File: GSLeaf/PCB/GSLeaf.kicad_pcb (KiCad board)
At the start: 2 copper layers, 30 x 103 mm, 119 parts, among them Q1 LED_5050, Q2 IRLML6401, Q3 IRLML6401, Q4 IRLML9303, Q5 2N7002, SW1 SWITCH, SW2 BTN, SW3 BTN, SW4 DIPx6

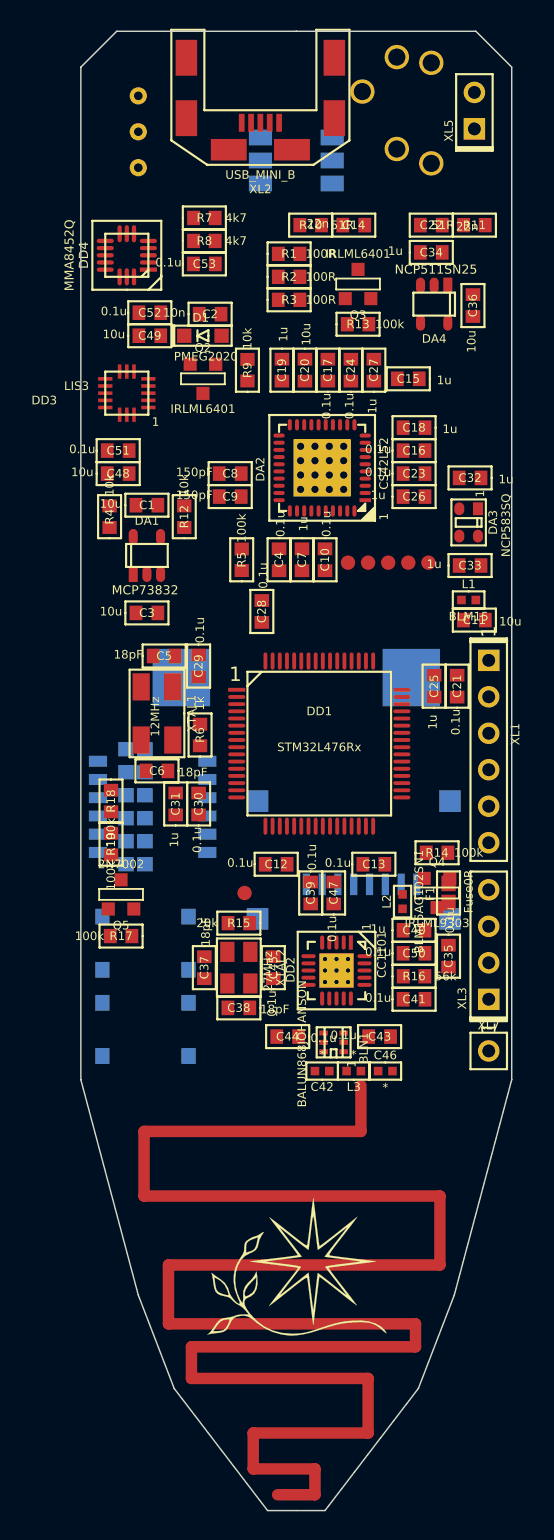
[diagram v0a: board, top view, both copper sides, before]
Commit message: Leaf sent to factory
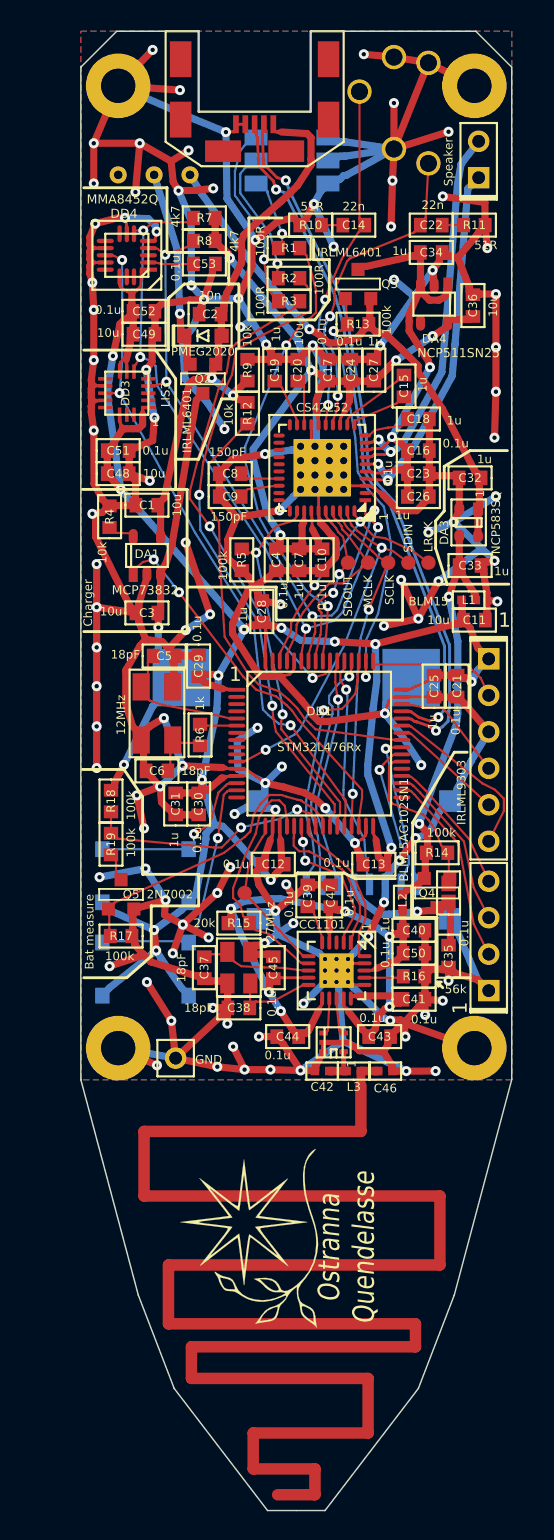
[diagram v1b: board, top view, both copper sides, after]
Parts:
- removed F2, F3, F4, F5, F6, F7: Fuse0R, Resistors:RES_0603_FUSE
- removed SW4: DIPx6, BtnsSwitches:DIP_SMD_1D27X6
- added HOLE1: HOLE_METALLED, PCB:Hole2d4_out4d5mm, F.Cu at (130.6, 61.8)
- added HOLE2: HOLE_METALLED, PCB:Hole2d4_out4d5mm, F.Cu at (130.6, 128.8)
- added HOLE3: HOLE_METALLED, PCB:Hole2d4_out4d5mm, F.Cu at (155.4, 61.8)
- added HOLE4: HOLE_METALLED, PCB:Hole2d4_out4d5mm, F.Cu at (155.4, 128.8)
- moved XL7 21.8 mm to (134.6, 129.5)
- moved R12 8.44 mm to (139.6, 84.6)
- moved SW2 4.70 mm to (132.5, 116.8), turned to 180 degrees
- moved SW3 4.20 mm to (132.5, 123.3)
- moved Logo1 3.81 mm to (139.7, 142.1), turned to 90 degrees
- moved XL5 3.41 mm to (155.7, 68.2)
- moved SW1 3.20 mm to (133.1, 68.0), turned to 180 degrees
- moved C18 0.67 mm to (151.5, 85.0)
- moved XL3 0.60 mm to (156.4, 124.8)
- moved C15 0.58 mm to (150.5, 82.7), turned to 90 degrees
- moved C19 0.50 mm to (141.5, 81.6)
- moved C20 0.50 mm to (143.1, 81.6)
- moved C49 0.41 mm to (132.4, 79.1)
- moved XL2 0.41 mm to (140.1, 63.6)
- moved C52 0.41 mm to (132.4, 77.5)
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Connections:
- DD1 pad 10: /DS1 -> (no net)
- DD1 pad 2: /DS6 -> (no net)
- DD1 pad 3: /DS5 -> (no net)
- DD1 pad 4: /DS4 -> (no net)
- DD1 pad 8: /DS3 -> (no net)
- DD1 pad 9: /DS2 -> (no net)
- Q1 pad 1: GND -> Net-(Q1-Pad1)
- Q1 pad 2: GND -> Net-(Q1-Pad2)
- Q1 pad 3: GND -> Net-(Q1-Pad3)
- Q1 pad 4: Net-(Q1-Pad4) -> GND
- Q1 pad 5: Net-(Q1-Pad5) -> GND
- Q1 pad 6: Net-(Q1-Pad6) -> GND
- R1 pad 1: Net-(Q1-Pad6) -> Net-(Q1-Pad1)
- R2 pad 1: Net-(Q1-Pad5) -> Net-(Q1-Pad2)
- R3 pad 1: Net-(Q1-Pad4) -> Net-(Q1-Pad3)
- XL2 pad H2: Net-(XL2-PadH1) -> (no net)
- XL2 pad H3: Net-(XL2-PadH3) -> (no net)
- XL2 pad H4: Net-(XL2-PadH3) -> Net-(XL2-PadH4)
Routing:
- net GND: track 0.00 -> 648.1 mm, vias 0 -> 116
- net PwrMCU: track 0.00 -> 158.5 mm, vias 0 -> 13
- net /ANT2: track 0.00 -> 142.0 mm
- net VCC: track 0.00 -> 59.9 mm, vias 0 -> 6
- net VAA: track 0.00 -> 58.3 mm, vias 0 -> 5
- net /SDA: track 0.00 -> 51.0 mm, vias 0 -> 4
- net /D-: track 0.00 -> 48.4 mm, vias 0 -> 2
- net /D+: track 0.00 -> 47.4 mm, vias 0 -> 2
- net /SCL: track 0.00 -> 47.2 mm, vias 0 -> 4
- net /ACC_INT1: track 0.00 -> 46.7 mm, vias 0 -> 3
- net /RED_LED: track 0.00 -> 44.7 mm, vias 0 -> 2
- net /GREEN_LED: track 0.00 -> 42.7 mm, vias 0 -> 2
- net +5V: track 0.00 -> 40.4 mm, vias 0 -> 2
- net PwrUnst: track 0.00 -> 38.1 mm, vias 0 -> 1
- net /PWR_CTRLED: track 0.00 -> 32.7 mm, vias 0 -> 2
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- added copper zone on B.Cu, net GND
- added copper zone on F.Cu, net GND
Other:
- outline, holes or cut-outs redrawn
- net class Default: clearance 0.2 -> 0.15; trace_width 0.25 -> 0.15; via_dia 0.8 -> 0.7; via_drill 0.4 -> 0.3
- net class Wide added: clearance 0.15, trace_width 0.5, via_dia 0.7, via_drill 0.3
- rule pad_to_mask_clearance: 0 -> 0.1
- rule trace_clearance: 0.2 -> 0.15
- rule trace_min: 0.2 -> 0.1
- board text added: "+"
- board text added: "-"
- board text added: "Bat measure"
- board text added: "Charger"
- board text added: "GND"
- board text added: "LRCK"
- board text added: "MCLK"
- board text added: "Off On"
- board text added: "Ostranna Quendelasse"
- board text added: "PB13"
- board text added: "PB14"
- board text added: "PB15"
- board text added: "SCLK"
- board text added: "SDIN"
- board text added: "SDOUT"
- board text added: "Speaker"

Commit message: New leaf sch nearly ready
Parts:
- removed ANT1: ANT_PCB_MONO, Radio:ANT_868_SEIDHE
- removed B1: BAT, Installation:EEMB603030
- removed BLN1: BALUN868JOHANSON, Radio:BALUN_JOHANSON868
- removed C1, C11, C20, C3, C36, C48, C49: 10u, Capacitors:CAP_0603
- removed C10, C12, C13, C16, C17, C21, C23, C24, C28, C29, C30, C35, C39, C4, C41, C43, C44, C45, C47, C50, C51, C52, C53: 0.1u, Capacitors:CAP_0603
- removed C14, C22: 22n, Capacitors:CAP_0603
- removed C15, C18, C19, C25, C26, C27, C31, C32, C33, C34, C40, C7: 1u, Capacitors:CAP_0603
- removed C2: 10n, Capacitors:CAP_0603
- removed C37, C38, C5, C6: 18pF, Capacitors:CAP_0603
- removed C42, C46: *, Capacitors:CAP_0402
- removed C8, C9: 150pF, Capacitors:CAP_0603
- removed D1: PMEG2020, Diodes:SOD323
- removed DA1: MCP73832, SOT:SOT23-5
- removed DA2: CS42L52, QFN_DFN:QFN40
- removed DA3: NCP583SQ, SOT:SC82AB
- removed DA4: NCP511SN25, SOT:SOT23-5
- removed DD1: STM32L476Rx, LQFP_TQFP:LQFP64
- removed DD2: CC1101, QFN_DFN:QFN20
- removed DD3: LIS3, LGA:LGA16_3X3_5_3
- removed DD4: MMA8452Q, QFN_DFN:QFN16_5x3
- removed F1: Fuse0R, Resistors:RES_0603_FUSE
- removed HOLE1, HOLE2, HOLE3, HOLE4: HOLE_METALLED, PCB:Hole2d4_out4d5mm
- removed L1: BLM15, Inductors:IND_0402
- removed L2: BLM15AG102SN1, Inductors:IND_0402
- removed L3: *, Inductors:IND_0402
- removed Logo1: Logo, Pictures:Ostranna_12d7_10d1
- removed Q1: LED_5050, LEDs:LED_5050
- removed Q2, Q3: IRLML6401, SOT:SOT23-3
- removed Q4: IRLML9303, SOT:SOT23-3
- removed Q5: 2N7002, SOT:SOT23-3
- removed R1, R2, R3: 100R, Resistors:RES_0603
- removed R10, R11: 51R, Resistors:RES_0603
- removed R12, R4, R9: 10k, Resistors:RES_0603
- removed R13, R14, R17, R18, R19, R5: 100k, Resistors:RES_0603
- removed R15: 20k, Resistors:RES_0603
- removed R16: 56k, Resistors:RES_0603
- removed R6: 1k, Resistors:RES_0603
- removed R7, R8: 4k7, Resistors:RES_0603
- removed SW1: SWITCH, BtnsSwitches:SW_SS-1P2T
- removed SW2, SW3: BTN, BtnsSwitches:BTN_4x4_SMD
- removed TP2, TP3, TP4, TP5, TP6, TP7: TESTPOINT, PCB:TESTPOINT_1MM
- removed XL1: CONN_6, Connectors:PLS-6
- removed XL2: USB_MINI_B, Connectors:USBmicro_MOLEX_WM17142
- removed XL3: CONN_4, Connectors:PLS-4
- removed XL4: AudioJackSimple, Connectors:AUDIO_CKX3_5_30
- removed XL5: CONN_2, Connectors:PLS-2
- removed XL6: CONN_MICROSD, Connectors:MICROSD_CAP_FIX05A
- removed XL7: CONN_1, Connectors:PLS-1Rnd
- removed XTAL1: 12MHz, Quartz:0503x4-4
- removed XTAL2: 27MHz, Quartz:03225C4
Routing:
- net GND: track 648.1 -> 0.00 mm, vias 116 -> 0
- net PwrMCU: track 158.5 -> 0.00 mm, vias 13 -> 0
- net /ANT2: track 142.0 -> 0.00 mm
- net VCC: track 59.9 -> 0.00 mm, vias 6 -> 0
- net VAA: track 58.3 -> 0.00 mm, vias 5 -> 0
- net /SDA: track 51.0 -> 0.00 mm, vias 4 -> 0
- net /D-: track 48.4 -> 0.00 mm, vias 2 -> 0
- net /D+: track 47.4 -> 0.00 mm, vias 2 -> 0
- net /SCL: track 47.2 -> 0.00 mm, vias 4 -> 0
- net /ACC_INT1: track 46.7 -> 0.00 mm, vias 3 -> 0
- net /RED_LED: track 44.7 -> 0.00 mm, vias 2 -> 0
- net /GREEN_LED: track 42.7 -> 0.00 mm, vias 2 -> 0
- net +5V: track 40.4 -> 0.00 mm, vias 2 -> 0
- net PwrUnst: track 38.1 -> 0.00 mm, vias 1 -> 0
- net /PWR_CTRLED: track 32.7 -> 0.00 mm, vias 2 -> 0
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- removed copper zone on B.Cu, net GND
- removed copper zone on F.Cu, net GND
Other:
- board outline removed
- board text removed: "+"
- board text removed: "-"
- board text removed: "Bat measure"
- board text removed: "Charger"
- board text removed: "GND"
- board text removed: "LRCK"
- board text removed: "MCLK"
- board text removed: "Off On"
- board text removed: "Ostranna Quendelasse"
- board text removed: "PB13"
- board text removed: "PB14"
- board text removed: "PB15"
- board text removed: "SCLK"
- board text removed: "SDIN"
- board text removed: "SDOUT"
- board text removed: "Speaker"
